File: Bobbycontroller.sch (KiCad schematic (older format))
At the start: 37 parts, among them J1 Conn_01x01_Male, J11 Conn_01x01, J12 Conn_01x01, J13 Conn_01x01, J14 Conn_01x01, J15 -BATT, J16 +BATT, J2 Conn_01x01_Male, J3 Conn_01x01_Male, J5 Conn_01x01_Male, J6 Conn_01x01_Male, J7 Conn_01x01_Male

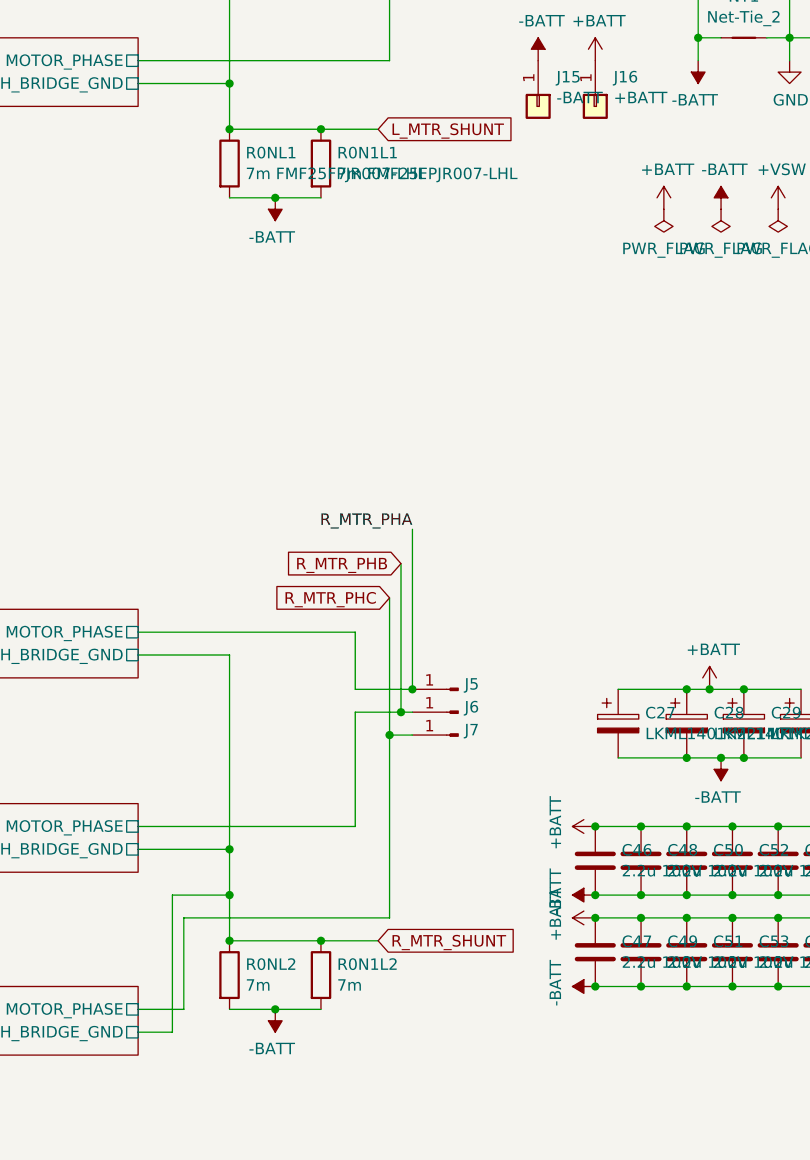
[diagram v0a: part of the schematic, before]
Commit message: add resistors on mosfet driver inputs, change board corners, fix labels
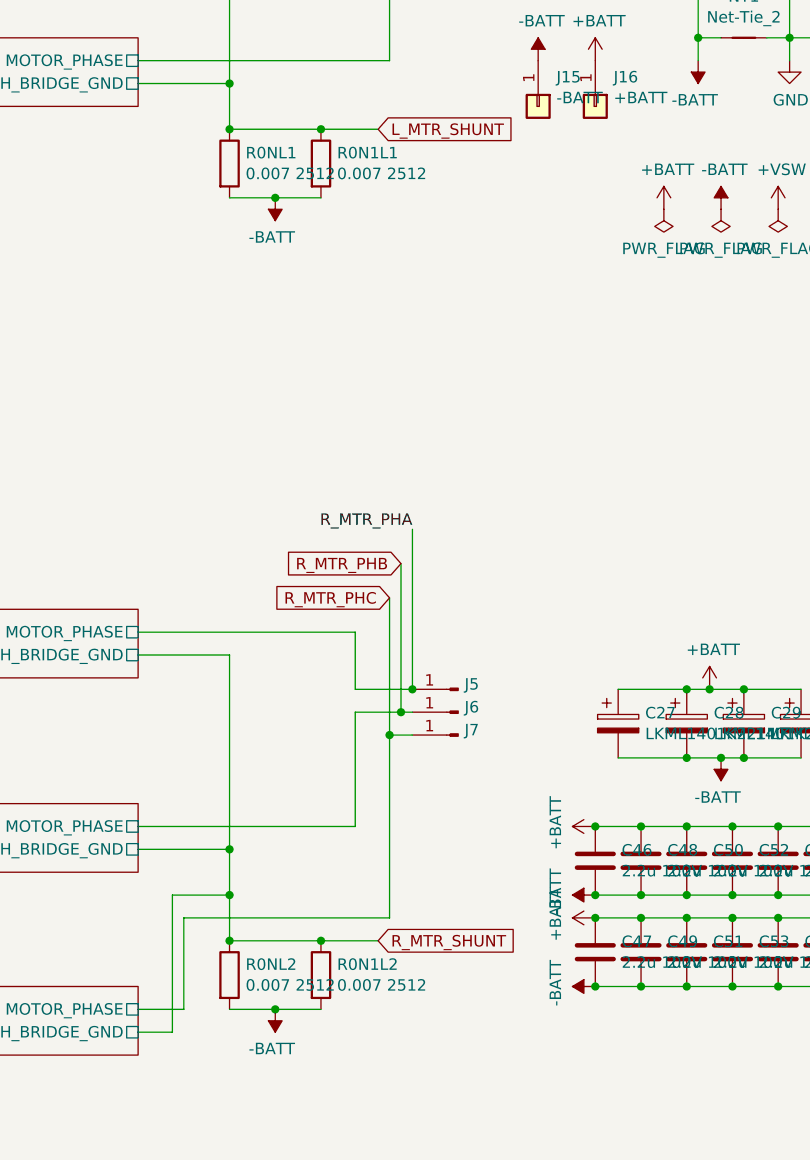
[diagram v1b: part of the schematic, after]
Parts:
- R0N1L1, R0NL1: value 7m FMF25FPJR007-LHL -> 0.007 2512
- R0N1L2, R0NL2: value 7m -> 0.007 2512
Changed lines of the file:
@@
 P 8500 2650
 F 0 "R0N1L1" H 8570 2696 50  0000 L CNN
-F 1 "7m FMF25FPJR007-LHL" H 8570 2605 50  0000 L CNN
+F 1 "0.007 2512" H 8570 2605 50  0000 L CNN
 F 2 "Resistor_SMD:R_2512_6332Metric" V 8430 2650 50  0001 C CNN
 F 3 "~" H 8500 2650 50  0001 C CNN
@@
 P 8100 2650
 F 0 "R0NL1" H 8170 2696 50  0000 L CNN
-F 1 "7m FMF25FPJR007-LHL" H 8170 2605 50  0000 L CNN
+F 1 "0.007 2512" H 8170 2605 50  0000 L CNN
 F 2 "Resistor_SMD:R_2512_6332Metric" V 8030 2650 50  0001 C CNN
 F 3 "~" H 8100 2650 50  0001 C CNN
@@
 P 8500 6200
 F 0 "R0N1L2" H 8570 6246 50  0000 L CNN
-F 1 "7m" H 8570 6155 50  0000 L CNN
+F 1 "0.007 2512" H 8570 6155 50  0000 L CNN
 F 2 "Resistor_SMD:R_2512_6332Metric" V 8430 6200 50  0001 C CNN
 F 3 "~" H 8500 6200 50  0001 C CNN
@@
 P 8100 6200
 F 0 "R0NL2" H 8170 6246 50  0000 L CNN
-F 1 "7m" H 8170 6155 50  0000 L CNN
+F 1 "0.007 2512" H 8170 6155 50  0000 L CNN
 F 2 "Resistor_SMD:R_2512_6332Metric" V 8030 6200 50  0001 C CNN
 F 3 "~" H 8100 6200 50  0001 C CNN
